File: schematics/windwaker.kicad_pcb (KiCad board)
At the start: 2 copper layers, 2 parts, among them U1 WEMOS_C3_mini, U2 TFT Display

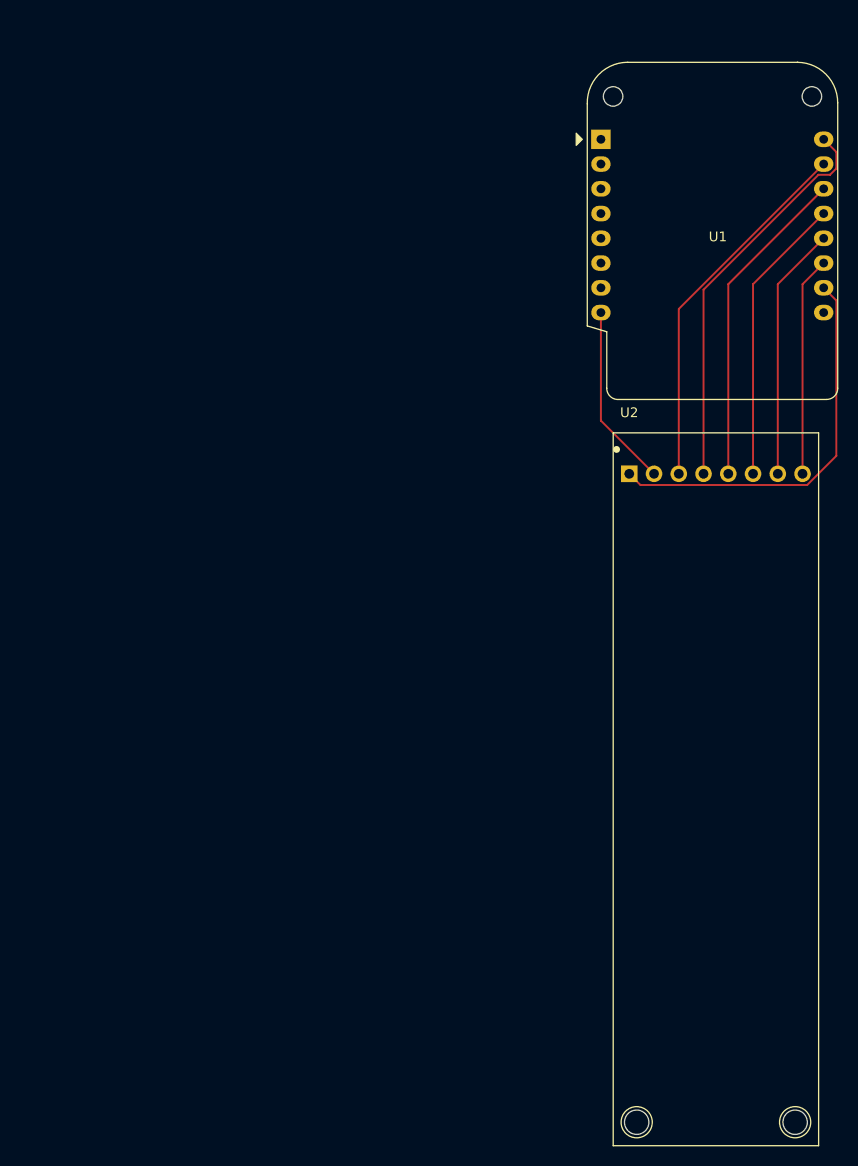
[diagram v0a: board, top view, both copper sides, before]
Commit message: adding some 3d models and routing the pcb
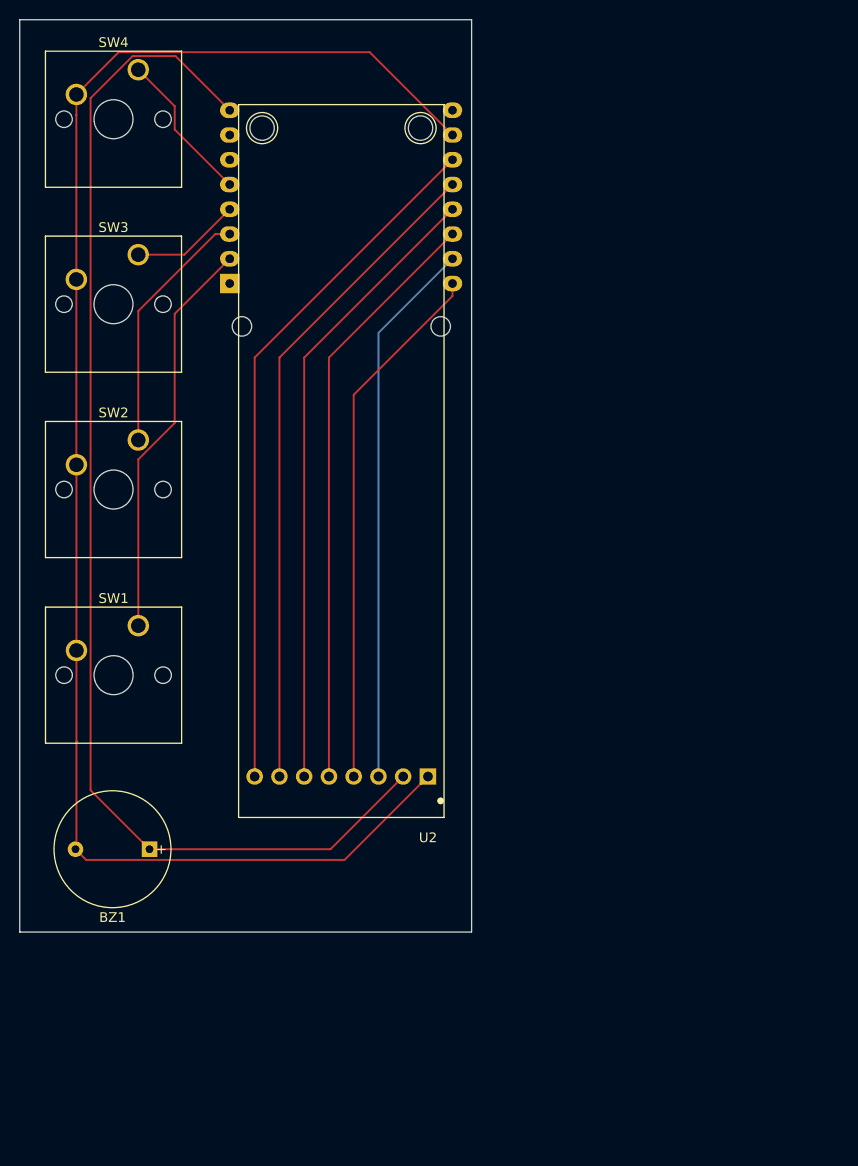
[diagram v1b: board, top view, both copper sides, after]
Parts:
- added BZ1: Buzzer, my_custom_library:Buzzer_12x9.5RM7.6, F.Cu at (87.3, 153.2)
- added SW1: SW_Push, Button_Switch_Keyboard:SW_Cherry_MX_1.00u_PCB, F.Cu at (90.0, 130.3)
- added SW2: SW_Push, Button_Switch_Keyboard:SW_Cherry_MX_1.00u_PCB, F.Cu at (90.0, 111.3)
- added SW3: SW_Push, Button_Switch_Keyboard:SW_Cherry_MX_1.00u_PCB, F.Cu at (90.0, 92.2)
- added SW4: SW_Push, Button_Switch_Keyboard:SW_Cherry_MX_1.00u_PCB, F.Cu at (90.0, 73.3)
- U1: moved to B.Cu
- moved U1 40.9 mm to (99.4, 95.2)
- moved U2 37.3 mm to (119.7, 145.8), turned to 180 degrees
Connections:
- U1 pad 3: unconnected-(U1-D2-Pad3) -> Net-(U1-D2)
- U1 pad 4: unconnected-(U1-D1-Pad4) -> Net-(U1-D1)
- U1 pad 5: unconnected-(U1-D0-Pad5) -> Net-(U1-D0)
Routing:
- net GND: track 40.7 -> 161.7 mm
- net +3V3: track 18.8 -> 127.1 mm
- net Net-(U1-D6): track 22.5 -> 71.7 mm
- net Net-(U1-D7): track 26.1 -> 68.1 mm
- net Net-(U1-D3): track 0.00 -> 41.5 mm
- net Net-(U1-D8): track 29.7 -> 64.5 mm
- net Net-(U1-D10): track 33.3 -> 60.9 mm
- net Net-(U1-D2): track 0.00 -> 25.9 mm
- net Net-(U1-RX): track 37.9 -> 56.3 mm
- net Net-(U1-D0): track 0.00 -> 15.7 mm
- net Net-(U1-TX): track 41.2 -> 54.8 mm
- net Net-(U1-D1): track 0.00 -> 11.3 mm
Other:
- board outline added: 46.4 x 93.6 mm
